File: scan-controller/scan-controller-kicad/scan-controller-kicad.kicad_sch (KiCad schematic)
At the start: 37 parts, among them CN1 24V in, J1 FTDI, J5 ICSP, J6 Raspi UART, J7 Raspi GPIO, Q2 IRLML2502, Q3 IRLML6402, SW3 Reset, U5 ATmega328P, Y1 8MHz

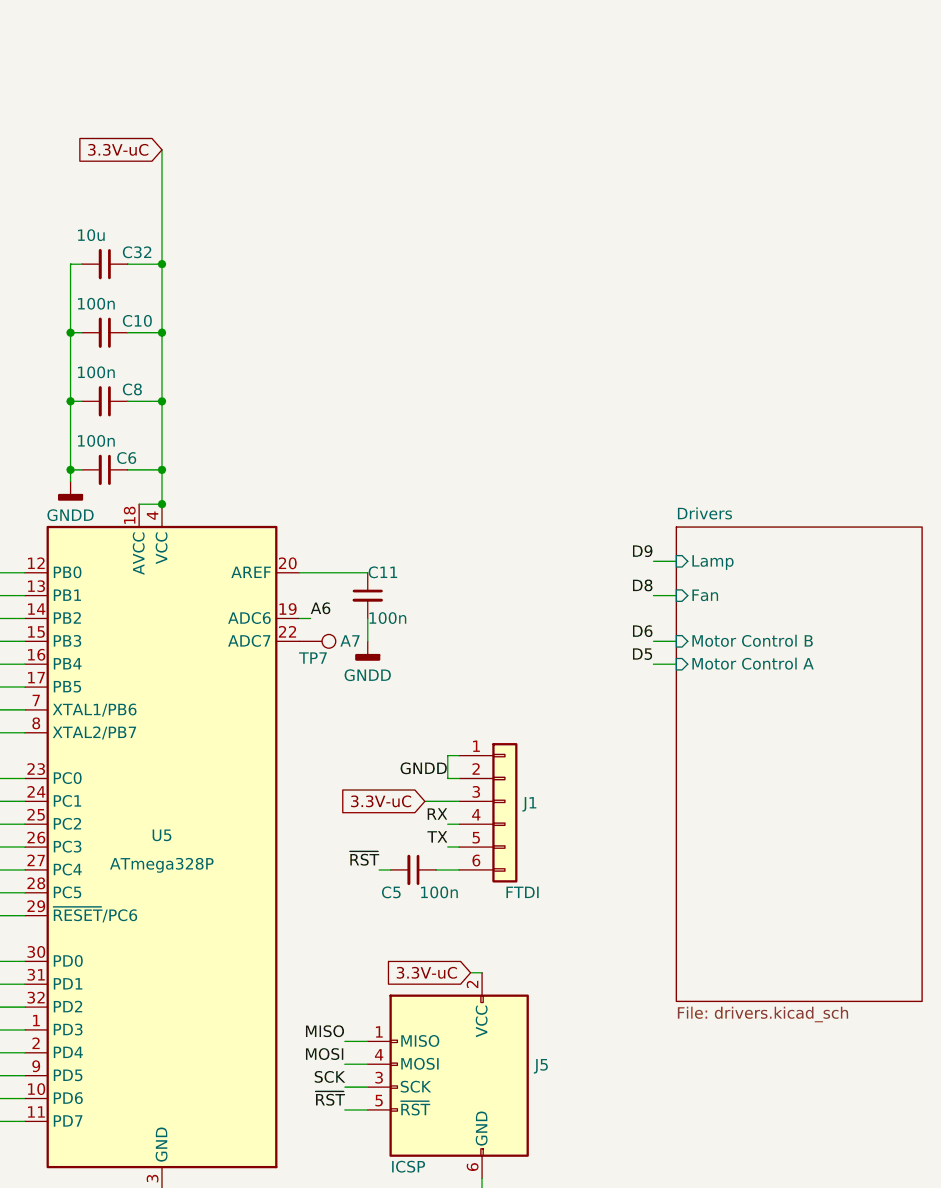
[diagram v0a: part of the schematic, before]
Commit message: Added Board Revision Detector
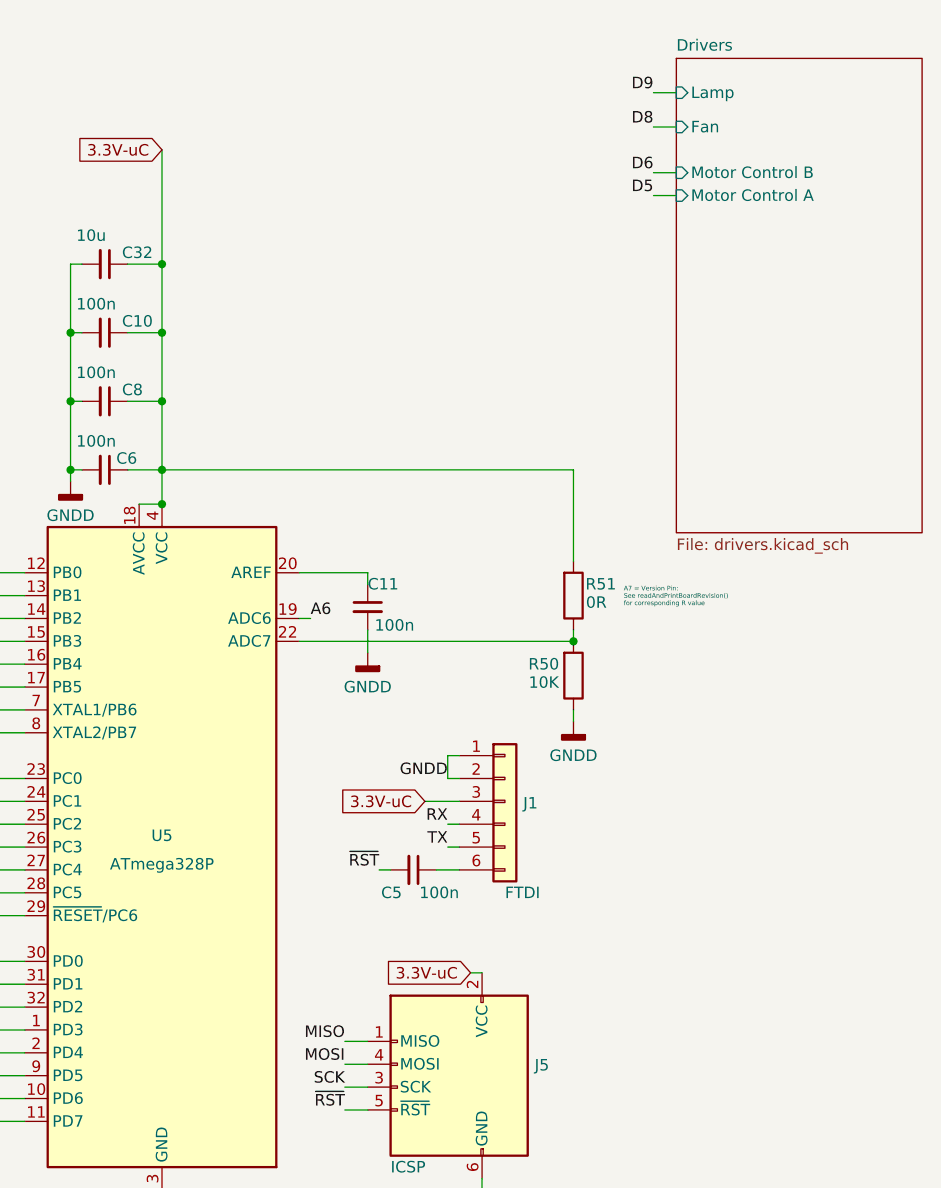
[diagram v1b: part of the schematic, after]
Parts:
- removed TP7: A7, Peacemans_Teile:TestPoint_THTPad_1.5x1.5mm_Drill0.7mm_named, symbol Peacemans_Teile:TestPoint_named
- added R50: 10K, Resistor_SMD:R_0805_2012Metric, symbol Device:R
- added R51: 0R, Resistor_SMD:R_0805_2012Metric, symbol Device:R
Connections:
- net 3.3V-uC: now also R51.2
- net GND: now also R50.1
- net at U5.22 (ADC7): now also R50.2, R51.1
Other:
- note added: "A7 = Version Pin: See readAndPrintBoardRevision() for corresponding R value"
- moved on the sheet: C11

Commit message: All better caps, more suitabel LDO for 50-> 5V
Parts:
- C32: footprint Capacitor_SMD:C_0805_2012Metric -> Capacitor_SMD:C_1210_3225Metric; LCSC C15850 -> C5156756
- C4: LCSC C90272 -> C487135
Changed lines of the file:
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@@
 			)
 		)
-		(property "Description" ""
+		(property "Description" "22pF 50V C0G"
 			(at 158.75 92.71 0)
 			(effects
@@
 			)
 		)
-		(property "Description" ""
+		(property "Description" "22pF 50V C0G"
 			(at 158.75 97.79 0)
 			(effects
@@
 			)
 		)
-		(property "Description" ""
+		(property "Description" "100V 100nF X7R"
 			(at 212.09 81.28 0)
 			(effects
@@
 			)
 		)
-		(property "Datasheet" "https://datasheet.lcsc.com/lcsc/2208091830_ROQANG-RVT1H471M1213_C90272.pdf"
+		(property "Datasheet" "https://jlcpcb.com/api/file/downloadByFileSystemAccessId/8589039600370769920"
 			(at 48.26 31.75 0)
 			(effects
@@
 			)
 		)
-		(property "Description" ""
+		(property "Description" "470u 63V"
 			(at 48.26 31.75 0)
 			(effects
@@
 			)
 		)
-		(property "LCSC" "C90272"
+		(property "LCSC" "C487135"
 			(at 48.26 31.75 0)
 			(effects
@@
 			)
 		)
-		(property "Description" ""
+		(property "Description" "100V 100nF X7R"
 			(at 217.17 110.49 0)
 			(effects
@@
 			)
 		)
-		(property "Description" ""
+		(property "Description" "100V 100nF X7R"
 			(at 182.88 66.04 0)
 			(effects
@@
 			)
 		)
-		(property "Description" ""
+		(property "Description" "100V 100nF X7R"
 			(at 182.88 50.8 0)
 			(effects
@@
 			)
 		)
-		(property "Footprint" "Capacitor_SMD:C_0805_2012Metric"
+		(property "Footprint" "Capacitor_SMD:C_1210_3225Metric"
 			(at 182.88 43.18 0)
 			(effects
@@
 			)
 		)
-		(property "Datasheet" "https://datasheet.lcsc.com/lcsc/2304140030_Samsung-Electro-Mechanics-CL21B104KCFNNNE_C28233.pdf"
+		(property "Datasheet" "https://datasheet.lcsc.com/lcsc/2209061730_PSA-Prosperity-Dielectrics-FS32X106K101EGG_C5156756.pdf"
 			(at 182.88 43.18 0)
 			(effects
@@
 			)
 		)
-		(property "Description" ""
+		(property "Description" "10u 100V X7R"
 			(at 182.88 43.18 0)
 			(effects
@@
 			)
 		)
-		(property "LCSC" "C15850"
+		(property "LCSC" "C5156756"
 			(at 182.88 43.18 0)
 			(effects
@@
 			)
 		)
-		(property "Description" ""
+		(property "Description" "34u 10V X5R"
 			(at 115.57 91.44 0)
 			(effects
@@
 			)
 		)
-		(property "Description" ""
+		(property "Description" "100V 100nF X7R"
 			(at 121.92 91.44 0)
 			(effects
@@
 			)
 		)
-		(property "Description" ""
+		(property "Description" "100V 100nF X7R"
 			(at 182.88 58.42 0)
 			(effects
